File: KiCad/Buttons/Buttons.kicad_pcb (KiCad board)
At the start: 2 copper layers, 38.4 x 23.6 mm, 15 parts, among them J1 KEYB, SW1 SET, SW2 OK, SW3 UP, SW4 RHT, SW5 DWN, SW6 LFT

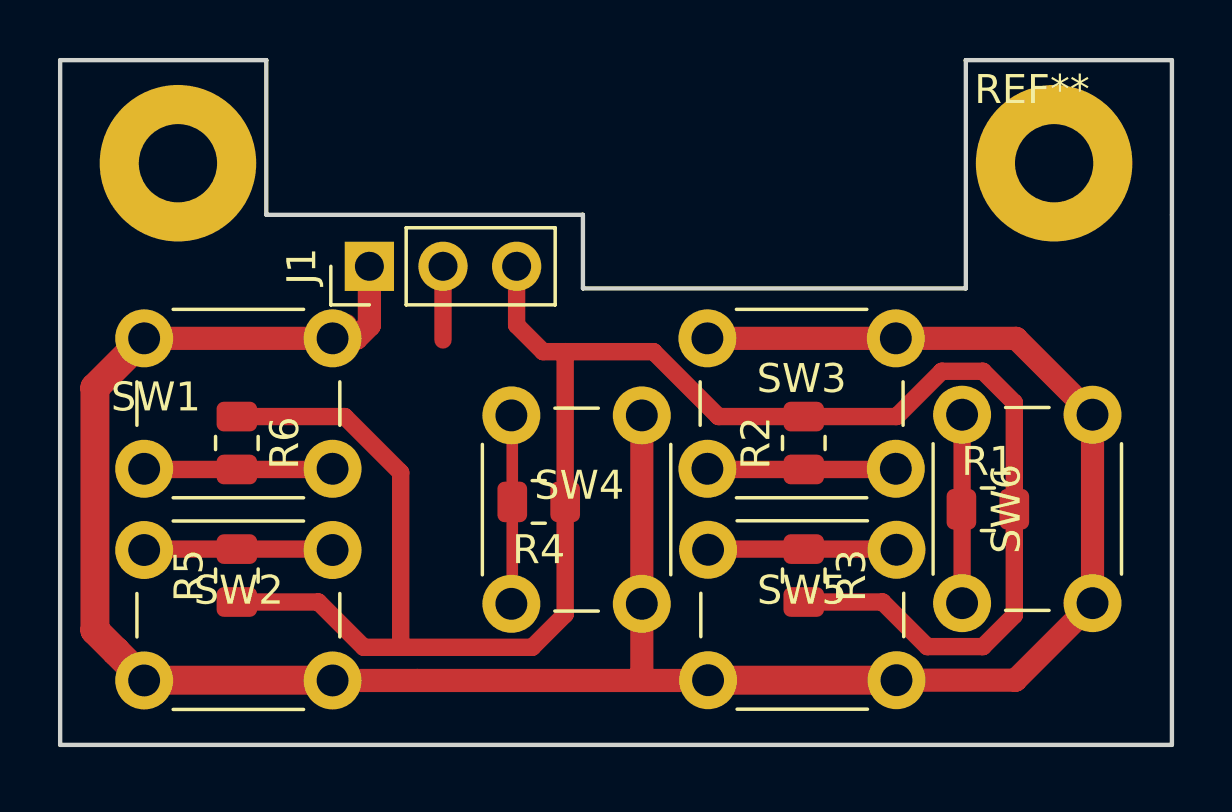
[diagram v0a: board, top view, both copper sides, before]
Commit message: Update
Update
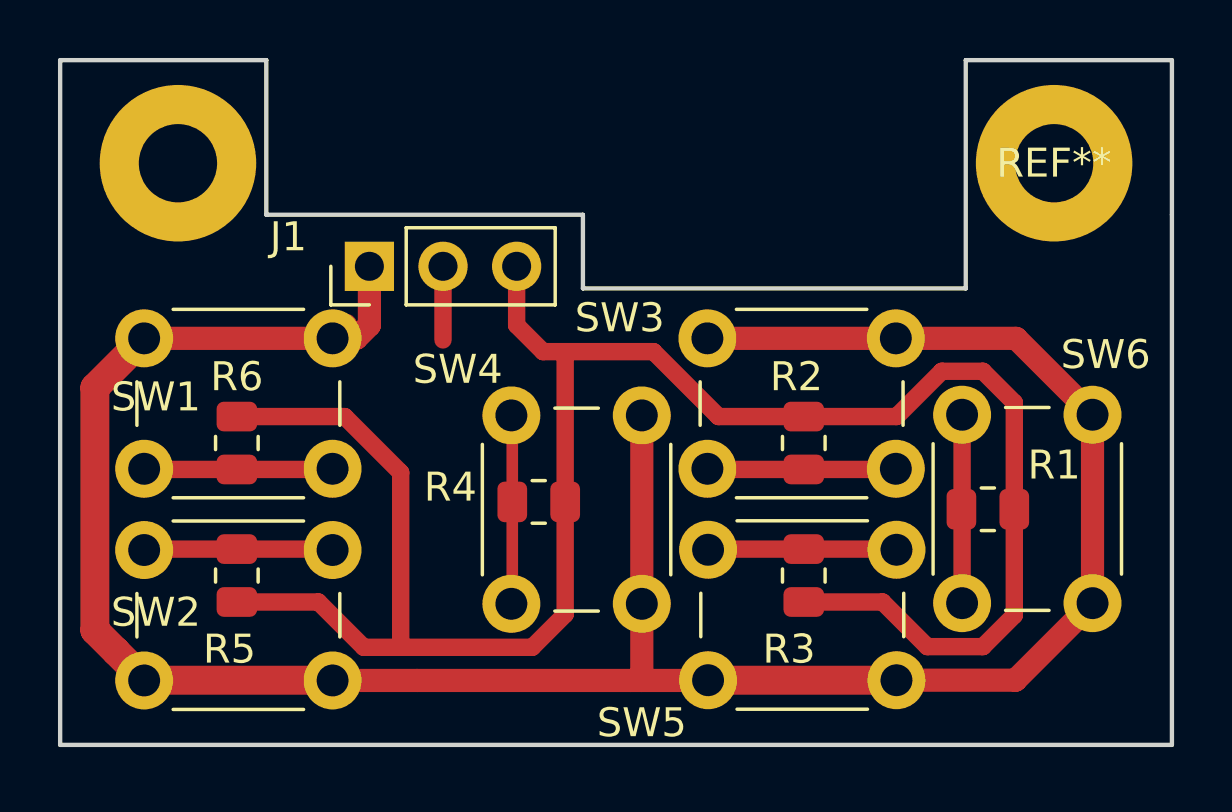
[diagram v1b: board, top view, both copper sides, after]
